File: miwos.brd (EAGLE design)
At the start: 120 x 120 mm, 51 parts, among them P1 MOUNT_CH, P2 MOUNT_CH, P3 MOUNT_CH, P4 MOUNT_CH

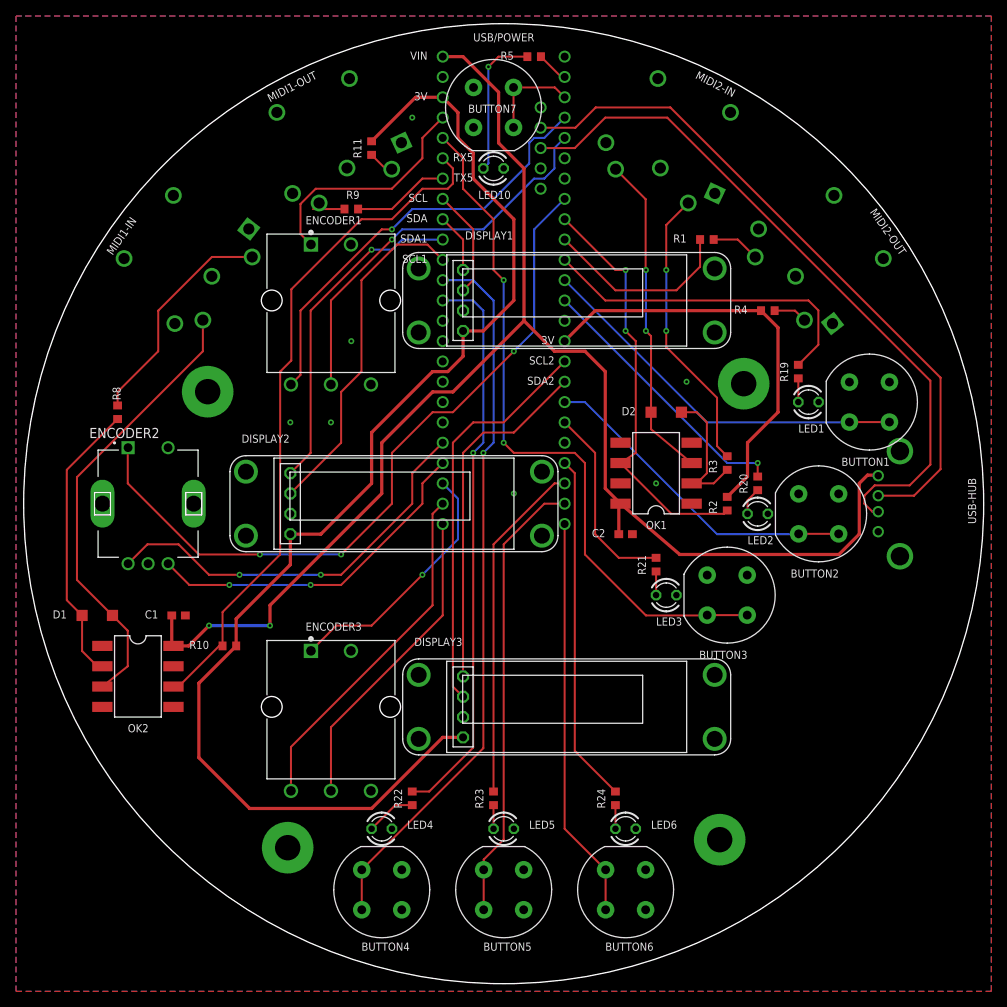
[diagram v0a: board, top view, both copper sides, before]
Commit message: Use TRS midi
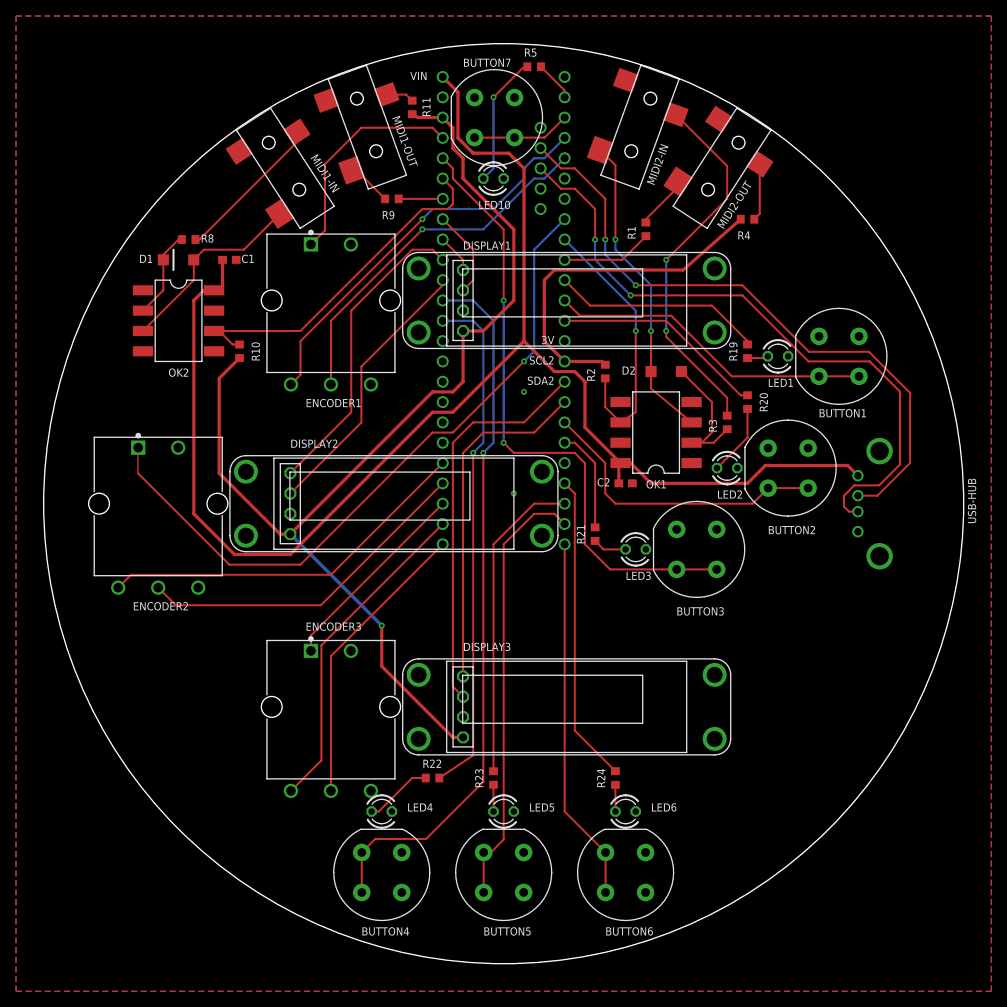
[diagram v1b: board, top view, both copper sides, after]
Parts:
- removed P1, P2, P3, P4: MOUNT_CH, sol_pin:MOUNT_CH32
- ENCODER2: value PEC11R-4215F-S0024 -> PEC16; device PEC11R-4215F-S0024:XDCR_PEC11R-4215F-S0024 -> PEC16:PEC16
- MIDI1-IN, MIDI1-OUT, MIDI2-IN, MIDI2-OUT: value ADAFRUIT-5PIN-DIN -> 35RASMT2BHNTRX; device adafruit-5pin-din:ADAFRUIT-5PIN-DIN -> 35RASMT2BHNTRX:SWITCHCRAFT_35RASMT2BHNTRX
- moved D1 45.6 mm to (-40.6, 30.5)
- moved C1 44.9 mm to (-34.3, 30.5)
- moved OK2 44.7 mm to (-40.6, 22.9)
- moved R10 36.9 mm to (-33.0, 19.1), turned to 90 degrees
- moved R8 23.3 mm to (-39.4, 33.0), turned to 180 degrees
- moved R2 22.5 mm to (12.7, 16.5)
- moved MIDI1-IN 16.8 mm to (-27.5, 42.2), flipped to the top, turned to 303 degrees
- moved MIDI2-OUT 16.8 mm to (27.5, 42.2), flipped to the top, turned to 237 degrees
- moved R4 11.7 mm to (30.5, 35.6)
- moved R20 10.2 mm to (30.5, 12.7)
- moved R21 8.52 mm to (11.4, -3.81)
- moved R1 7.73 mm to (17.8, 34.3), turned to 270 degrees
- moved R11 7.18 mm to (-11.4, 49.5), turned to 270 degrees
- moved BUTTON1 6.87 mm to (41.9, 18.4)
- moved BUTTON3 6.87 mm to (24.1, -5.71)
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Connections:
- net GND: now also ENCODER2.C, MIDI1-OUT.5, MIDI2-OUT.5; no longer ENCODER2.COM, MIDI1-IN.G1, MIDI1-IN.G2, MIDI1-OUT.2, MIDI1-OUT.G1, MIDI1-OUT.G2, MIDI2-IN.G1, MIDI2-IN.G2, MIDI2-OUT.2, MIDI2-OUT.G1, MIDI2-OUT.G2
- net N$10: now also MIDI1-IN.1; no longer MIDI1-IN.4
- net N$11: now also MIDI1-OUT.4; no longer MIDI1-OUT.5
- net N$12: now also MIDI1-OUT.1; no longer MIDI1-OUT.4
- net N$17: now also MIDI2-IN.4; no longer MIDI2-IN.5
- net N$18: now also MIDI2-IN.1; no longer MIDI2-IN.4
- net N$19: now also MIDI2-OUT.4; no longer MIDI2-OUT.5
- net N$21: now also MIDI2-OUT.1; no longer MIDI2-OUT.4
- net N$9: now also MIDI1-IN.4; no longer MIDI1-IN.5
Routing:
- net RX5: track 85.7 -> 44.0 mm
- net N$9: track 56.5 -> 24.7 mm
- net +3V3: track 210.8 -> 180.7 mm, vias 0 -> 1
- net N$8: track 35.7 -> 11.2 mm
- net RX2: track 52.1 -> 33.9 mm, vias 2 -> 1
- net BUTTON1-LED: track 42.2 -> 26.4 mm
- net TX2: track 24.2 -> 11.4 mm
- net BUTTON3-LED: track 24.4 -> 12.9 mm
- net N$18: track 35.9 -> 46.6 mm
- net BUTTON3: track 87.4 -> 77.9 mm
- net N$10: track 28.5 -> 19.0 mm
- net SCL1: track 43.1 -> 34.6 mm
- net BUTTON2-LED: track 34.2 -> 26.7 mm, vias 1 -> 0
- net BUTTON1: track 48.0 -> 40.7 mm
- net ENCODER3-PUSH: track 31.9 -> 25.2 mm, vias 1 -> 0
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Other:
- board size 120 x 120 mm -> 115 x 115 mm
- board text removed: "MIDI1-IN"
- board text removed: "MIDI1-OUT"
- board text removed: "MIDI2-IN"
- board text removed: "MIDI2-OUT"
- board text removed: "RX5"
- board text removed: "SCL"
- board text removed: "SCL1"
- board text removed: "SDA"
- board text removed: "SDA1"
- board text removed: "TX5"
- board text removed: "USB/POWER"
